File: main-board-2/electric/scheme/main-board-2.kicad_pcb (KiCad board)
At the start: 2 copper layers, 85 x 56 mm, 125 parts, among them K1 power-switch, K2 usb-power-switch, P1 batt, P10 rst, P11 screw-1, P13 screw-2, P14 gpio-big, P15 gpio-small, P16 moto-1, P17 moto-2, P2 CONN_4, P3 trigger-btn, P4 CONN_3X2, P5 reg-short-to-gnd-1, P6 reg-short-to-gnd-2, P7 bootloader, P8 cross board conn, P9 rst, Q1 IRLML2244, Q10 IRLML2244, Q11 sot223, Q12 bc857, Q13 irlml2244, Q2 BC847, Q3 IRLML2244, Q4 IRLML2244, Q5 BC847, Q6 BC847, Q7 BC847, Q8 BC847, Q9 IRLML2244, U1 LM317AEMP, U2 LM317AT, U3 LM317AEMP, U4 LM317AT, U5 LM293, U6 L298, U7 MINI-USB-B, X1 8MHz

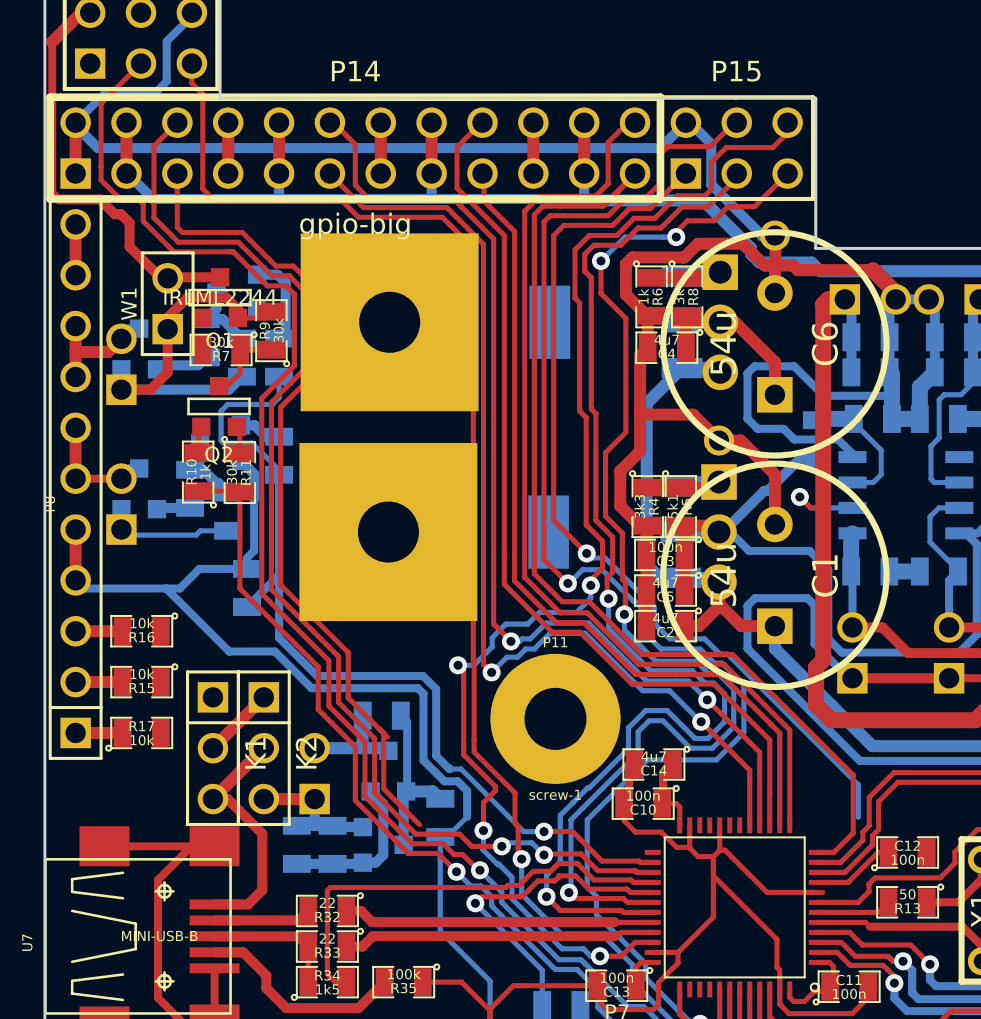
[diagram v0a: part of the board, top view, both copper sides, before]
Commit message: Routing...
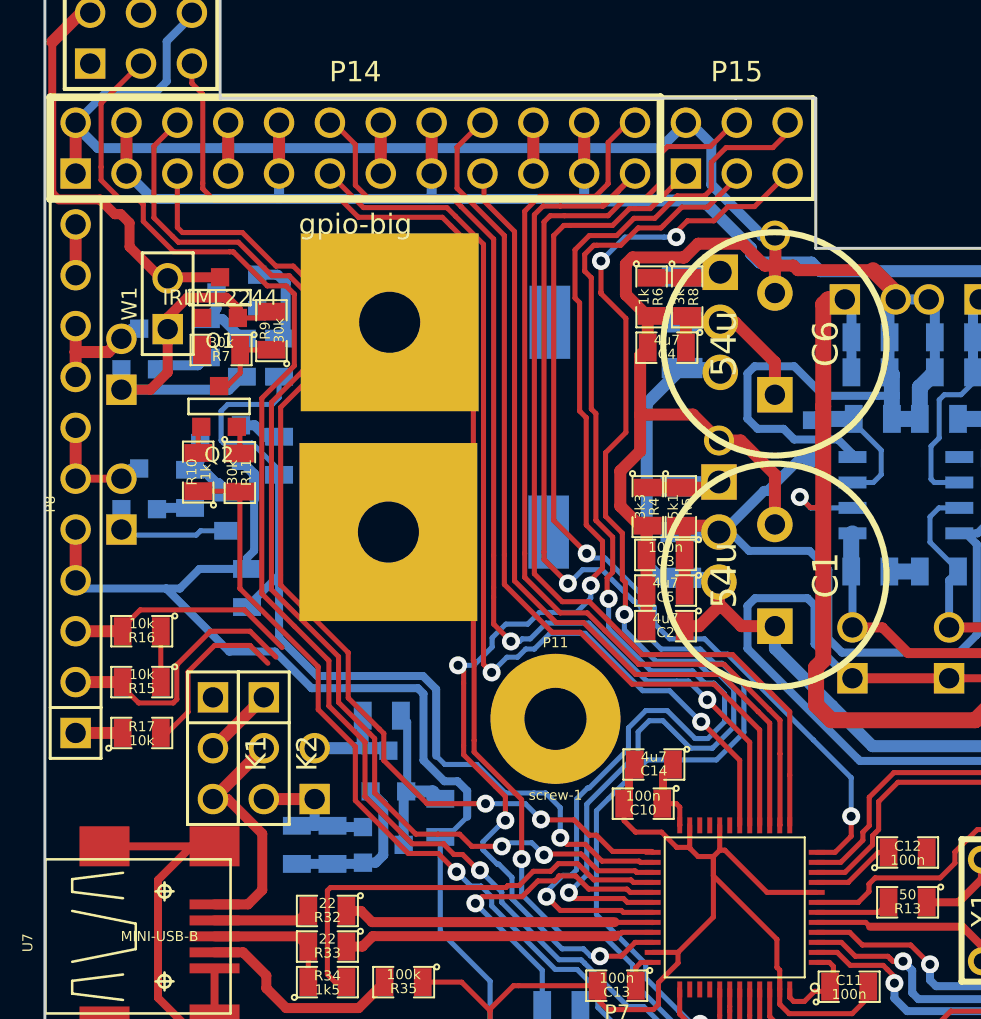
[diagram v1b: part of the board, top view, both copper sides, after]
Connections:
- stm1 pad 12: /gpio-4 -> /gpio-9
- stm1 pad 13: /gpio-8 -> /gpio-4
- stm1 pad 14: /gpio-3 -> /gpio-8
- stm1 pad 15: /gpio-7 -> /gpio-3
- stm1 pad 16: /gpio-6 -> /gpio-7
- stm1 pad 17: /gpio-2 -> /gpio-6
- stm1 pad 18: /gpio-1 -> /gpio-2
- stm1 pad 25: /gpio-9 -> /gpio-1
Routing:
- net /sda-int: track 2.35 -> 13.6 mm
- net /gpio-1: track 41.7 -> 52.5 mm, vias 0 -> 2
- net /scl-int: track 2.35 -> 11.6 mm
- net /addon-trigger: track 0.00 -> 8.70 mm
- net /gpio-4: track 51.3 -> 47.4 mm
- net /gpio-9: track 44.9 -> 47.7 mm, vias 1 -> 2
- net /addon-vdd: track 5.93 -> 8.47 mm
- net /addon-pwr-en: track 45.1 -> 46.0 mm
